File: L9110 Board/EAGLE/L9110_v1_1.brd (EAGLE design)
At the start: 90 x 90 mm, 46 parts, among them IC5 MCP23017SP, X4 057-016-0

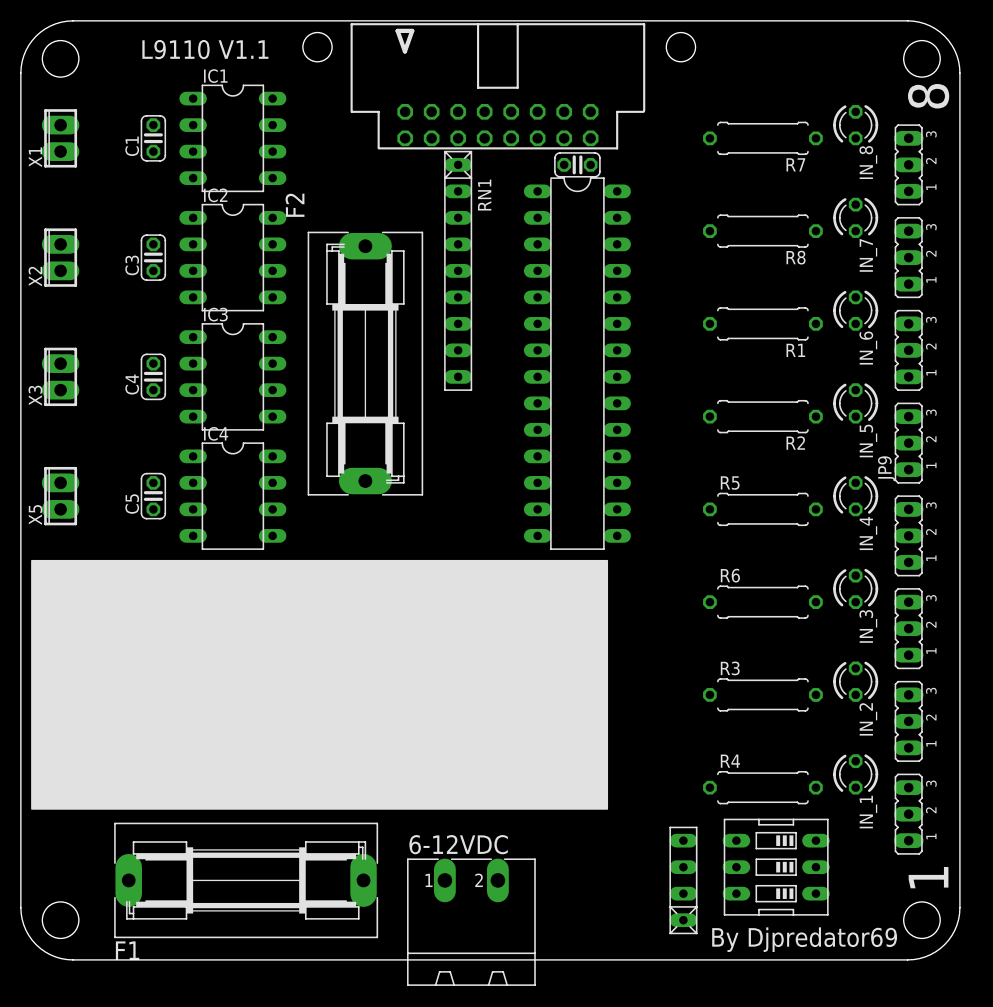
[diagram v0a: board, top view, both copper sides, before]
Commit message: Update L9110_v1_1.brd
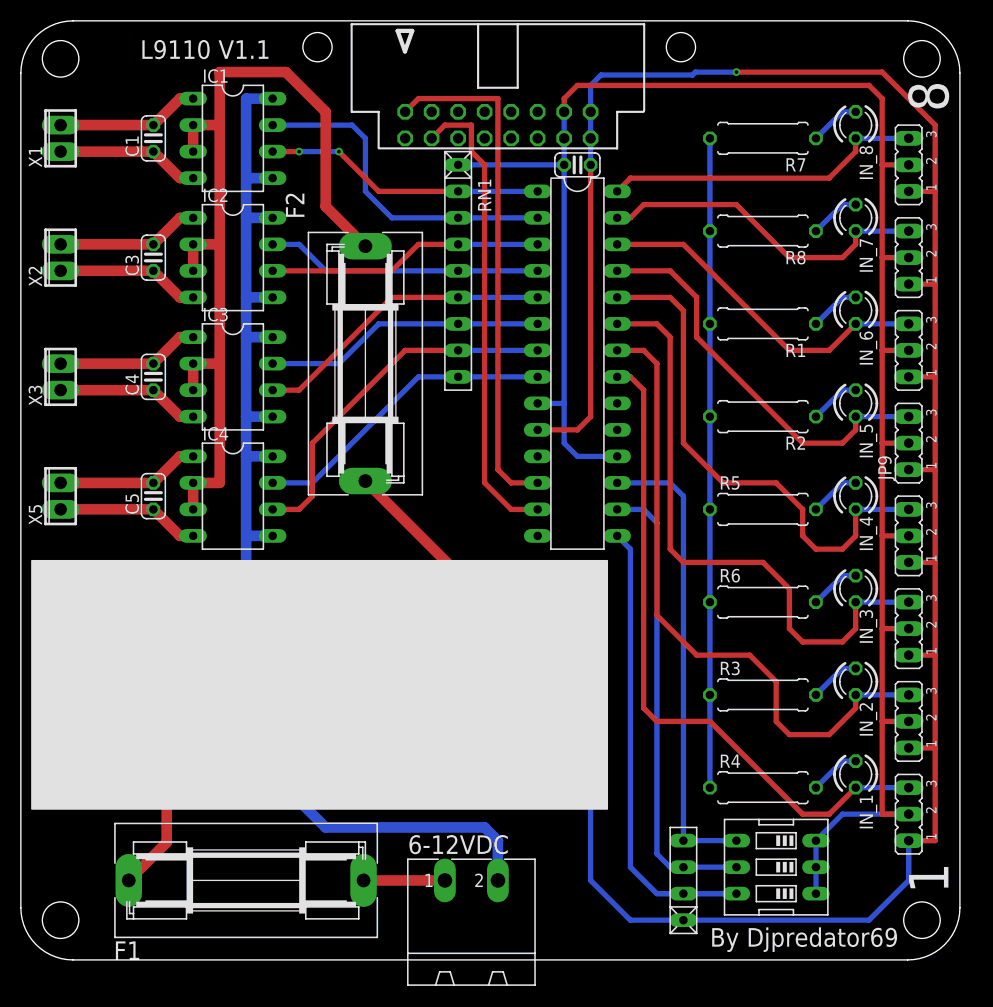
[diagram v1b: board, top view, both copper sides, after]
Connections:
- net GND2: now also U$2.OUTB-
- net N$37: now also U$2.INB+
- net N$38: now also U$2.INB-
- net N$39: now also U$2.OUTB+
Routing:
- net GND2: track 0.00 -> 322.9 mm, vias 0 -> 1
- net VCC5.1: track 0.00 -> 186.8 mm
- net N$18: track 0.00 -> 85.9 mm
- net N$21: track 0.00 -> 64.2 mm
- net VCC5.2: track 0.00 -> 62.2 mm
- net N$2: track 0.00 -> 61.9 mm
- net N$23: track 0.00 -> 57.8 mm
- net N$4: track 0.00 -> 49.9 mm
- net N$38: track 0.00 -> 49.8 mm
- net N$82: track 0.00 -> 49.3 mm
- net N$84: track 0.00 -> 45.3 mm
- net N$6: track 0.00 -> 45.0 mm
- net N$35: track 0.00 -> 44.2 mm
- net N$85: track 0.00 -> 43.5 mm
- net N$25: track 0.00 -> 38.8 mm
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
